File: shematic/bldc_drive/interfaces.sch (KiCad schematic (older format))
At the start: 11 parts, among them J2 Conn_01x04_Male, J4 Conn_01x02_Male, J5 Conn_01x02_Male, U10 TJA1051T, U11 MAX481E, U12 SN74AUP1T34DCK, U13 SN74AUP1T34DCK

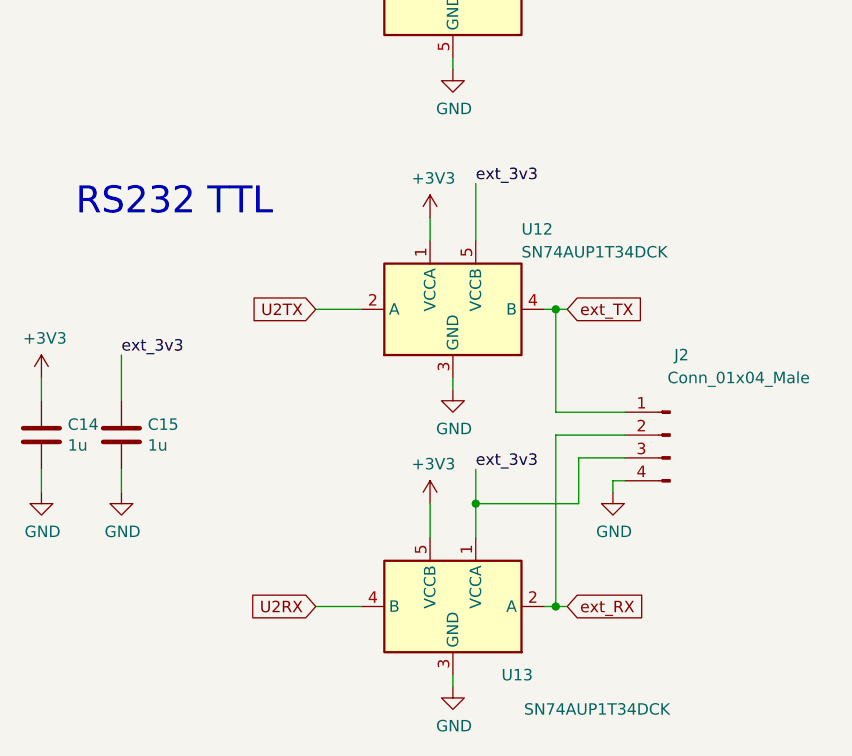
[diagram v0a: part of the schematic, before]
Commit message: --
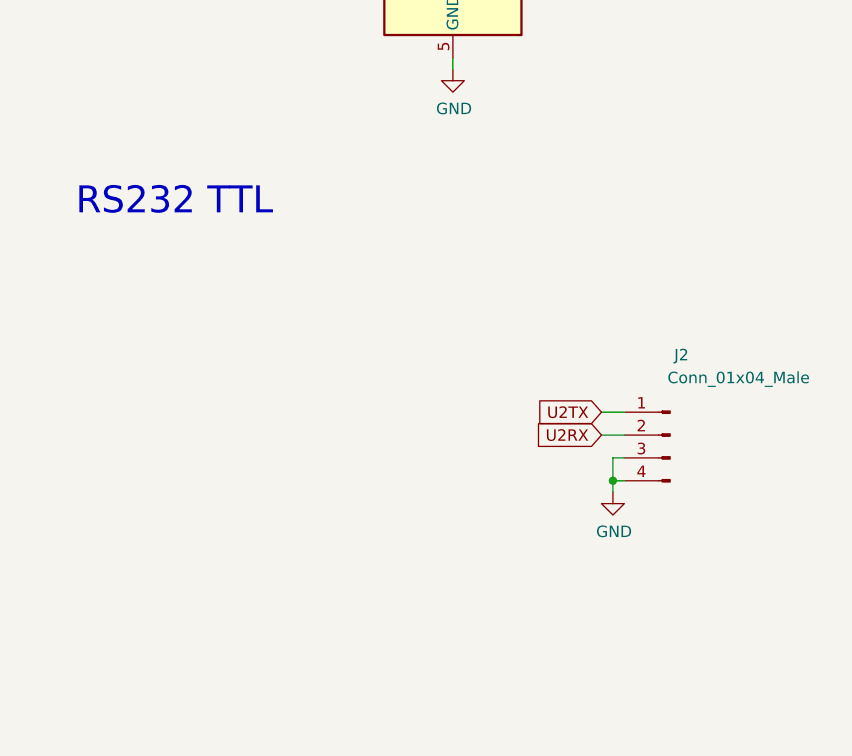
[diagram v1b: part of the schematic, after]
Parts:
- removed C14, C15: 1u, Capacitor_SMD:C_0805_2012Metric, symbol Device:C
- removed U12, U13: SN74AUP1T34DCK, Package_TO_SOT_SMD:SOT-353_SC-70-5, symbol Logic_LevelTranslator:SN74AUP1T34DCK
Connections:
- net ext_3v3 is gone; now on net GND: J2.3 (Pin_3)
- net ext_RX is gone; now on net U2RX: J2.2 (Pin_2)
- net ext_TX is gone; now on net U2TX: J2.1 (Pin_1)
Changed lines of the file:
@@
-	1    0    0    -1
-$EndComp
-$Comp
-L Logic_LevelTranslator:SN74AUP1T34DCK U12
-U 1 1 5EB1CE3F
-P 3600 4900
-F 0 "U12" H 3900 5250 50  0000 L CNN
-F 1 "SN74AUP1T34DCK" H 3900 5150 50  0000 L CNN
-F 2 "Package_TO_SOT_SMD:SOT-353_SC-70-5" H 3600 4200 50  0001 C CNN
-F 3 "http://www.ti.com/lit/ds/symlink/sn74aup1t34.pdf" H 3600 4300 50  0001 C CNN
-	1    3600 4900
 	1    0    0    -1
 $EndComp
@@
 Wire Wire Line
 	3100 3250 3100 3300
-Wire Wire Line
-	3700 4600 3700 4350
-Text Label 3700 5600 0    50   ~ 0
-ext_3v3
-Text Label 3700 4350 0    50   ~ 0
-ext_3v3
-$Comp
-L power:+3V3 #PWR0153
-U 1 1 5EB26243
-P 3500 4500
-F 0 "#PWR0153" H 3500 4350 50  0001 C CNN
-F 1 "+3V3" H 3515 4673 50  0000 C CNN
-F 2 "" H 3500 4500 50  0001 C CNN
-F 3 "" H 3500 4500 50  0001 C CNN
-	1    3500 4500
-	1    0    0    -1
-$EndComp
-$Comp
-L power:+3V3 #PWR0154
-U 1 1 5EB269EF
-P 3500 5750
-F 0 "#PWR0154" H 3500 5600 50  0001 C CNN
-F 1 "+3V3" H 3515 5923 50  0000 C CNN
-F 2 "" H 3500 5750 50  0001 C CNN
-F 3 "" H 3500 5750 50  0001 C CNN
-	1    3500 5750
-	1    0    0    -1
-$EndComp
-Wire Wire Line
-	3500 4600 3500 4500
-$Comp
-L power:GND #PWR0155
-U 1 1 5EB277E9
-P 3600 6550
-F 0 "#PWR0155" H 3600 6300 50  0001 C CNN
-F 1 "GND" H 3605 6377 50  0000 C CNN
-F 2 "" H 3600 6550 50  0001 C CNN
-F 3 "" H 3600 6550 50  0001 C CNN
-	1    3600 6550
-	1    0    0    -1
-$EndComp
-$Comp
-L power:GND #PWR0156
-U 1 1 5EB28095
-P 3600 5250
-F 0 "#PWR0156" H 3600 5000 50  0001 C CNN
-F 1 "GND" H 3605 5077 50  0000 C CNN
-F 2 "" H 3600 5250 50  0001 C CNN
-F 3 "" H 3600 5250 50  0001 C CNN
-	1    3600 5250
-	1    0    0    -1
-$EndComp
-Wire Wire Line
-	3600 5250 3600 5200
-Text GLabel 4100 4900 2    50   Input ~ 0
-ext_TX
-Text GLabel 4100 6200 2    50   Input ~ 0
-ext_RX
-Wire Wire Line
-	4000 4900 4050 4900
-Text GLabel 3000 4900 0    50   Input ~ 0
+Text GLabel 4250 5350 0    50   Input ~ 0
 U2TX
-Text GLabel 3000 6200 0    50   Input ~ 0
+Text GLabel 4250 5450 0    50   Input ~ 0
 U2RX
-Wire Wire Line
-	3000 4900 3200 4900
 $Comp
 L Device:R R33
@@
 Wire Wire Line
 	2850 3100 3200 3100
-$Comp
-L Device:C C15
-U 1 1 5EB36166
-P 2150 5450
-F 0 "C15" H 2265 5496 50  0000 L CNN
-F 1 "1u" H 2265 5405 50  0000 L CNN
-F 2 "Capacitor_SMD:C_0805_2012Metric" H 2188 5300 50  0001 C CNN
-F 3 "~" H 2150 5450 50  0001 C CNN
-	1    2150 5450
-	1    0    0    -1
-$EndComp
-$Comp
-L Device:C C14
-U 1 1 5EB365C9
-P 1800 5450
-F 0 "C14" H 1915 5496 50  0000 L CNN
-F 1 "1u" H 1915 5405 50  0000 L CNN
-F 2 "Capacitor_SMD:C_0805_2012Metric" H 1838 5300 50  0001 C CNN
-F 3 "~" H 1800 5450 50  0001 C CNN
-	1    1800 5450
-	1    0    0    -1
-$EndComp
-$Comp
-L power:GND #PWR0157
-U 1 1 5EB3682B
-P 1800 5700
-F 0 "#PWR0157" H 1800 5450 50  0001 C CNN
-F 1 "GND" H 1805 5527 50  0000 C CNN
-F 2 "" H 1800 5700 50  0001 C CNN
-F 3 "" H 1800 5700 50  0001 C CNN
-	1    1800 5700
-	1    0    0    -1
-$EndComp
-$Comp
-L power:GND #PWR0158
-U 1 1 5EB36BF0
-P 2150 5700
-F 0 "#PWR0158" H 2150 5450 50  0001 C CNN
-F 1 "GND" H 2155 5527 50  0000 C CNN
-F 2 "" H 2150 5700 50  0001 C CNN
-F 3 "" H 2150 5700 50  0001 C CNN
-	1    2150 5700
-	1    0    0    -1
-$EndComp
-Wire Wire Line
-	2150 5700 2150 5600
-Wire Wire Line
-	1800 5700 1800 5600
-$Comp
-L power:+3V3 #PWR0159
-U 1 1 5EB37F65
-P 1800 5200
-F 0 "#PWR0159" H 1800 5050 50  0001 C CNN
-F 1 "+3V3" H 1815 5373 50  0000 C CNN
-F 2 "" H 1800 5200 50  0001 C CNN
-F 3 "" H 1800 5200 50  0001 C CNN
-	1    1800 5200
-	1    0    0    -1
-$EndComp
-Wire Wire Line
-	1800 5300 1800 5200
-Wire Wire Line
-	2150 5300 2150 5100
-Text Label 2150 5100 0    50   ~ 0
-ext_3v3
-$Comp
-L Logic_LevelTranslator:SN74AUP1T34DCK U13
-U 1 1 5EB1D336
-P 3600 6200
-F 0 "U13" H 3250 5900 50  0000 L CNN
-F 1 "SN74AUP1T34DCK" H 2650 5750 50  0000 L CNN
-F 2 "Package_TO_SOT_SMD:SOT-353_SC-70-5" H 3600 5500 50  0001 C CNN
-F 3 "http://www.ti.com/lit/ds/symlink/sn74aup1t34.pdf" H 3600 5600 50  0001 C CNN
-	1    3600 6200
-	-1   0    0    -1
-$EndComp
-Wire Wire Line
-	3700 5900 3700 5750
-Wire Wire Line
-	3500 5900 3500 5750
-Wire Wire Line
-	4000 6200 4050 6200
-Wire Wire Line
-	3600 6550 3600 6500
-Wire Wire Line
-	3000 6200 3200 6200
 Text Notes 1950 4500 0    118  ~ 0
 RS232 TTL
@@
 $EndComp
 Wire Wire Line
-	4050 5350 4050 4900
-Connection ~ 4050 4900
-Wire Wire Line
-	4050 4900 4100 4900
-Wire Wire Line
-	4050 5450 4050 6200
-Connection ~ 4050 6200
-Wire Wire Line
-	4050 6200 4100 6200
-Wire Wire Line
-	4350 5350 4050 5350
-Wire Wire Line
-	4350 5450 4050 5450
-Wire Wire Line
 	4300 5700 4300 5650
 Wire Wire Line
 	4300 5650 4350 5650
-Wire Wire Line
-	4350 5550 4150 5550
-Wire Wire Line
-	4150 5550 4150 5750
-Wire Wire Line
-	4150 5750 3700 5750
-Connection ~ 3700 5750
-Wire Wire Line
-	3700 5750 3700 5600
 $Comp
 L Connector:Conn_01x02_Male J4
@@
 Text Label 7300 2050 2    50   ~ 0
 RS485_A
+Wire Wire Line
+	4350 5550 4300 5550
+Wire Wire Line
+	4300 5550 4300 5650
+Connection ~ 4300 5650
+Wire Wire Line
+	4250 5450 4350 5450
+Wire Wire Line
+	4250 5350 4350 5350
 $EndSCHEMATC
